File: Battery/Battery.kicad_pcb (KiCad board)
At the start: 2 copper layers, 3 parts, among them J1 Conn_01x03_Pin, J2 Conn_01x05, J4 Conn_01x04

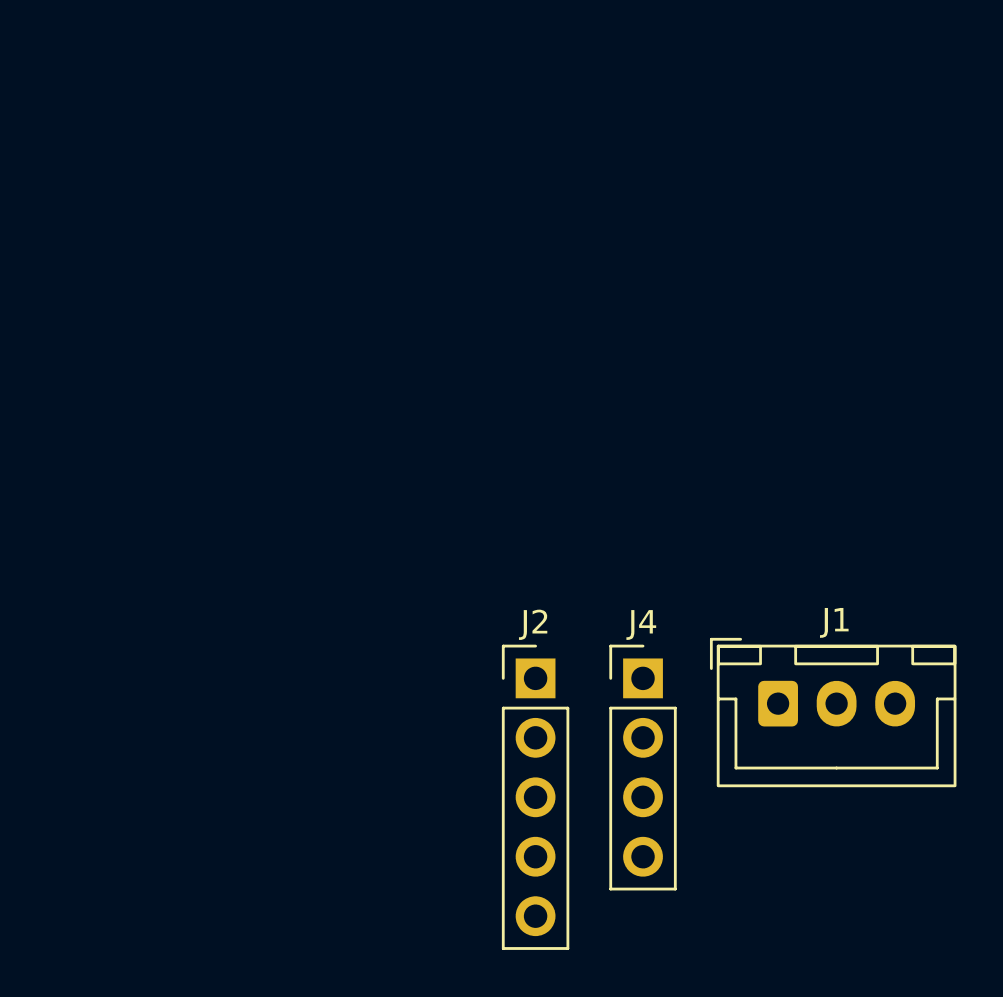
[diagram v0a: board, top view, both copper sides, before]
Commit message: Battery PCB
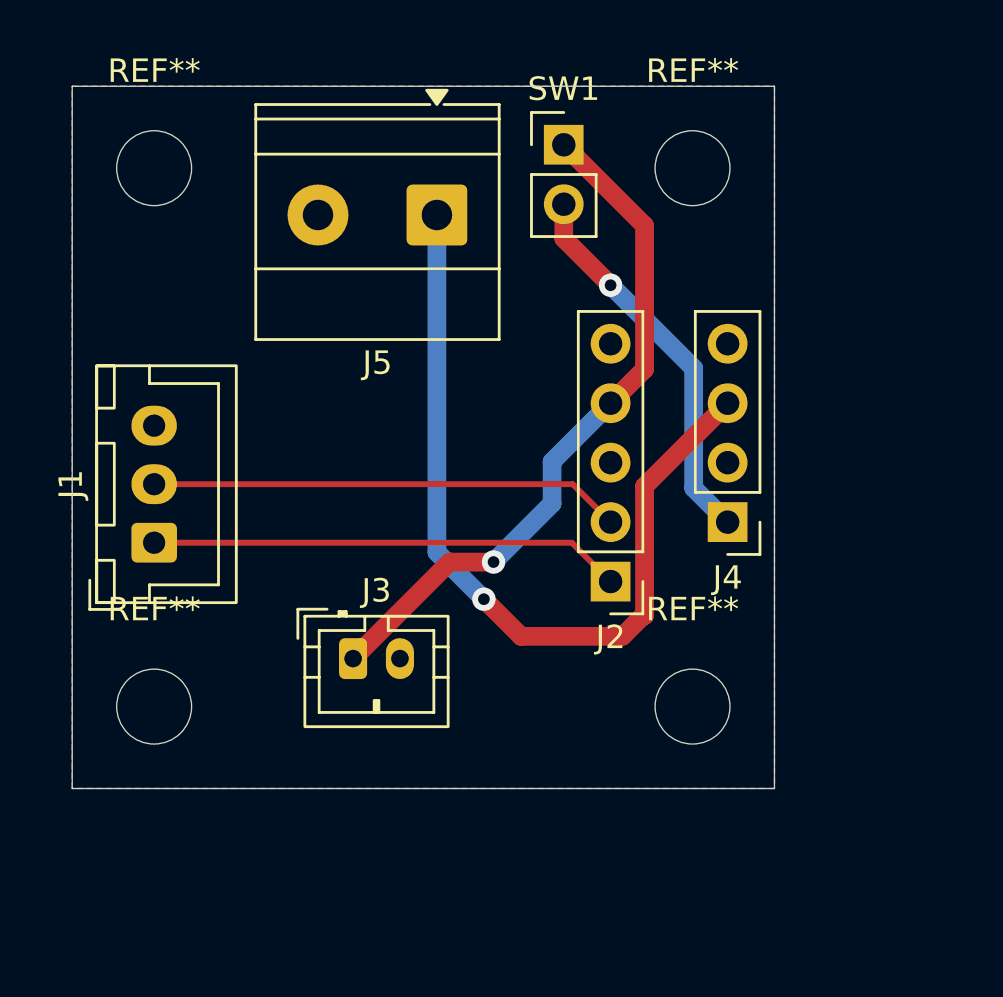
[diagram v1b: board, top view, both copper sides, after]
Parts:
- added J3: Conn_01x02, Connector_JST:JST_PH_B2B-PH-K_1x02_P2.00mm_Vertical, F.Cu at (24.0, 36.5)
- added J5: Conn_01x02, TerminalBlock_Phoenix:TerminalBlock_Phoenix_MKDS-1,5-2-5.08_1x02_P5.08mm_Horizontal, F.Cu at (27.6, 17.5)
- added REF**: MountingHole_3.2mm_M3, MountingHole:MountingHole_3.2mm_M3, F.Cu at (15.5, 15.5)
- added REF**: MountingHole_3.2mm_M3, MountingHole:MountingHole_3.2mm_M3, F.Cu at (15.5, 38.5)
- added REF**: MountingHole_3.2mm_M3, MountingHole:MountingHole_3.2mm_M3, F.Cu at (38.5, 15.5)
- added REF**: MountingHole_3.2mm_M3, MountingHole:MountingHole_3.2mm_M3, F.Cu at (38.5, 38.5)
- added SW1: SW_SPST, Connector_PinHeader_2.54mm:PinHeader_1x02_P2.54mm_Vertical, F.Cu at (33.0, 14.5)
- moved J1 27.5 mm to (15.5, 31.5), turned to 90 degrees
- moved J4 7.59 mm to (40.0, 30.6), turned to 180 degrees
- moved J2 5.23 mm to (35.0, 33.2), turned to 180 degrees
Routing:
- net +5V: track 0.00 -> 35.7 mm, vias 0 -> 1
- net VBATT: track 0.00 -> 29.6 mm, vias 0 -> 1
- net PACK_TOP: track 0.00 -> 20.2 mm
- net PACK_MID: track 0.00 -> 20.2 mm
- net VBATT_SW: track 0.00 -> 16.5 mm, vias 0 -> 1
- added copper zone on B.Cu, net GND
- added copper zone on F.Cu, net GND
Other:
- board outline added: 30 x 30 mm
